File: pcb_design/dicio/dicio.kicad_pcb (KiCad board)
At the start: 2 copper layers, 93 x 93 mm, 88 parts, among them J1 USB_OTG, J2 Conn_01x06_Female, J3 Screw_Terminal_01x06, J4 Screw_Terminal_01x11, J5 Conn_02x03_Odd_Even, J6 Screw_Terminal_01x05, J7 Screw_Terminal_01x09, P1 USB_C_Plug_USB2.0, SW1 SW_SPST, SW2 SW_SPST, SW3 SW_DIP_x08, U1 FT232RL, U2 MCP2542FD, U3 dsPIC33EP512MC806, U4 TPS737, U5 PCA9670, U6 TPS61040, U7 RP604x, U8 gloxinia_connector_small, Y1 Crystal_GND24

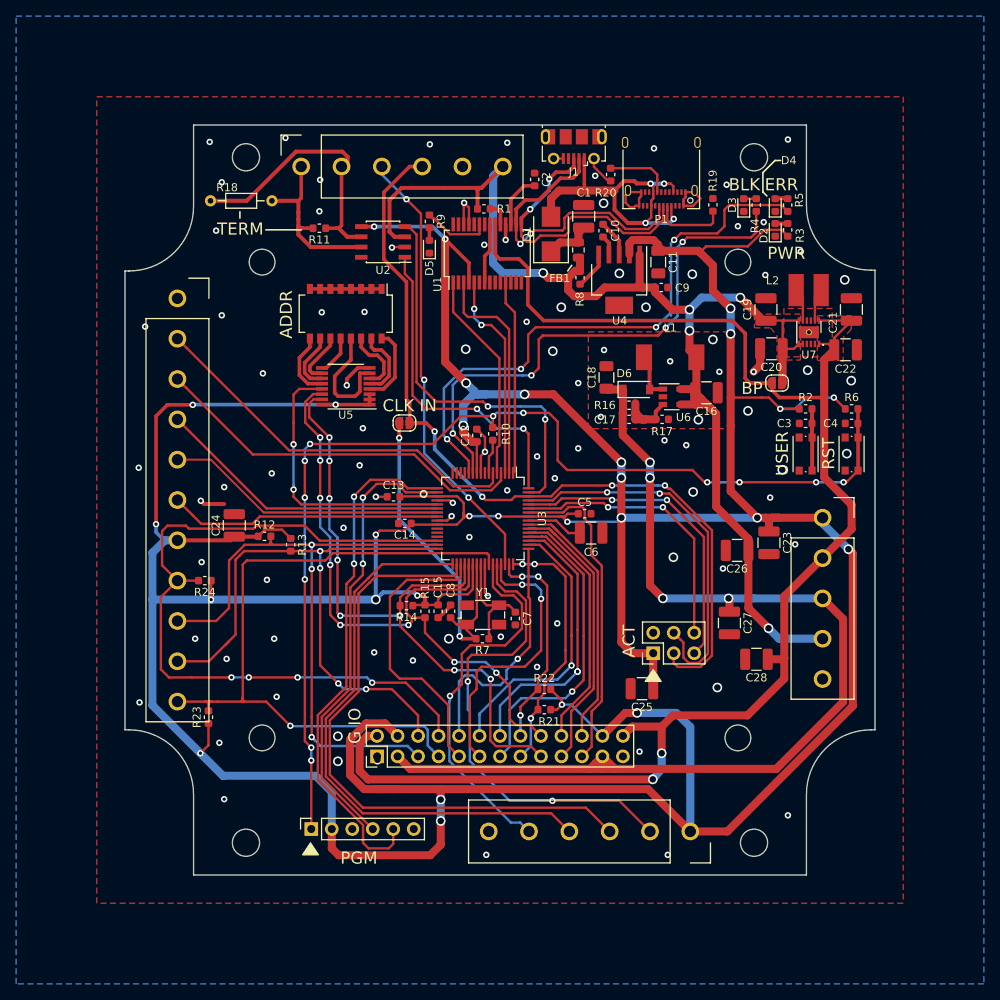
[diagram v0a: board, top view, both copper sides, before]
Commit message: New dicio design.
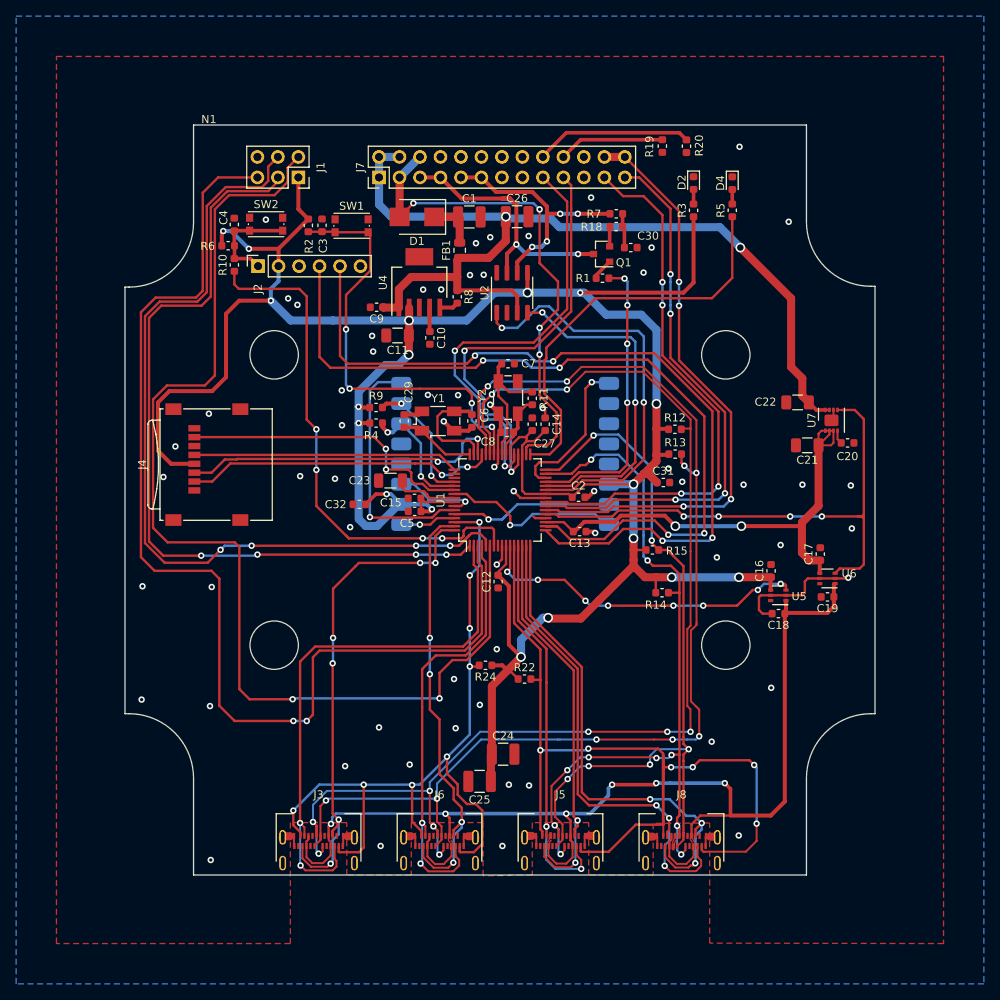
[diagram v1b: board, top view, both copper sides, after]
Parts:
- removed C28: 10uF, Capacitor_SMD:C_1210_3225Metric
- removed D3, D5: LED, LED_SMD:LED_0603_1608Metric
- removed D6: MBR0530, Diode_SMD:D_SOD-123
- removed H1, H2, H3, H4: MountingHole, MountingHole:MountingHole_3.2mm_M3
- removed JP1: Jumper_NC_Small, Jumper:SolderJumper-2_P1.3mm_Open_RoundedPad1.0x1.5mm
- removed JP2: Jumper, Jumper:SolderJumper-2_P1.3mm_Open_RoundedPad1.0x1.5mm
- removed L1: 10uH, custom_footprints:L_6.5mmx4.5mm_Bourns
- removed L2: 2.2uH, custom_footprints:L_L4mm_D4mm_H1.8mm
- removed P1: USB_C_Plug_USB2.0, custom_footprints:USB_C_Receptacle_Amphenol_12401832E402A
- removed R16: 1.8M, Capacitor_SMD:C_0603_1608Metric
- removed R17: 205k, Capacitor_SMD:C_0603_1608Metric
- removed R21, R23: 4.9k, Resistor_SMD:R_0603_1608Metric
- removed SW3: SW_DIP_x08, Button_Switch_SMD:SW_DIP_SPSTx08_Slide_Omron_A6H-8101_W6.15mm_P1.27mm
- removed U8: gloxinia_connector_small, Connector_PinHeader_2.54mm:PinHeader_2x13_P2.54mm_Vertical
- added C29: 20pF, Capacitor_SMD:C_0603_1608Metric, F.Cu at (73.1, 75.2)
- added C30: 4.7nF, Capacitor_SMD:C_0603_1608Metric, F.Cu at (101.2, 53.7)
- added C31: 0.1uF, Capacitor_SMD:C_0603_1608Metric, F.Cu at (105.2, 82.8)
- added C32: 0.1uF, Capacitor_SMD:C_0603_1608Metric, F.Cu at (67.6, 85.5)
- added J8: USB_C_Receptacle, custom_footprints:USB_C_Receptacle_Amphenol_12401861XX12A, F.Cu at (107.5, 127.9)
- added Q1: Q_NMOS_GSD, Package_TO_SOT_SMD:SOT-23, F.Cu at (97.6, 54.5)
- added Y2: Crystal_GND24, Crystal:Crystal_SMD_Abracon_ABM3B-4Pin_5.0x3.2mm, F.Cu at (86.0, 72.3)
- C16: value 10uF -> 1uF; footprint Capacitor_SMD:C_1210_3225Metric -> Capacitor_SMD:C_0603_1608Metric
- C17: value 4.7pF -> 1uF
- C18: value 1uF -> 0.1uF; footprint Capacitor_SMD:C_1206_3216Metric -> Capacitor_SMD:C_0603_1608Metric
- C19, C27: value 10uF -> 0.1uF; footprint Capacitor_SMD:C_1210_3225Metric -> Capacitor_SMD:C_0603_1608Metric
- C20: value 10uF -> 1nF; footprint Capacitor_SMD:C_1210_3225Metric -> Capacitor_SMD:C_0603_1608Metric
- C21, C22: value 22uF -> 4.7uF; footprint Capacitor_SMD:C_1210_3225Metric -> Capacitor_SMD:C_1206_3216Metric
- C23: footprint Capacitor_SMD:C_1210_3225Metric -> Capacitor_SMD:C_1206_3216Metric
- C6: value 10uF -> 20pF; footprint Capacitor_SMD:C_1210_3225Metric -> Capacitor_SMD:C_0603_1608Metric
- C7, C8: value 10pF -> 20pF
- J1: value USB_OTG -> Conn_02x03_Counter_Clockwise; footprint Connector_USB:USB_Micro-B_Molex-105017-0001 -> Connector_PinSocket_2.54mm:PinSocket_2x03_P2.54mm_Vertical
- J3: value Screw_Terminal_01x06 -> USB_C_Receptacle; footprint custom_footprints:TB003-500-06 -> custom_footprints:USB_C_Receptacle_Amphenol_12401861XX12A
- J4: value Screw_Terminal_01x11 -> Micro_SD_Card; footprint custom_footprints:TB003-500-11 -> Connector_Card:microSD_HC_Wuerth_693072010801
- J5: value Conn_02x03_Odd_Even -> USB_C_Receptacle; footprint Connector_PinHeader_2.54mm:PinHeader_2x03_P2.54mm_Vertical -> custom_footprints:USB_C_Receptacle_Amphenol_12401861XX12A
- J6: value Screw_Terminal_01x05 -> USB_C_Receptacle; footprint custom_footprints:TB003-500-05 -> custom_footprints:USB_C_Receptacle_Amphenol_12401861XX12A
- J7: value Screw_Terminal_01x09 -> Conn_02x13_Odd_Even; footprint custom_footprints:TB003-500-06 -> Connector_PinHeader_2.54mm:PinHeader_2x13_P2.54mm_Vertical
- N1: footprint custom_footprints:Enclosure-Hammond-1554LA -> custom_footprints:Enclosure-Gloxinia2
- R1: value 10k -> 1k
- R11: value 120 -> 1M
- R18: value 120R -> 60R; footprint Resistor_THT:R_Axial_DIN0204_L3.6mm_D1.6mm_P7.62mm_Horizontal -> Resistor_SMD:R_0603_1608Metric
- R4, R9: value 750 -> 100k
- R7: value 1M -> 60R
- SW1, SW2: footprint Button_Switch_SMD:SW_SPST_KMR2 -> Button_Switch_SMD:SW_Push_1P1T_NO_CK_KMR2
- U1: value FT232RL -> dsPIC33EP256MU806; footprint Package_SO:SSOP-28_5.3x10.2mm_P0.65mm -> Package_QFP:TQFP-64_10x10mm_P0.5mm
- U3: value dsPIC33EP512MC806 -> S70FL01GS; footprint Package_QFP:TQFP-64_10x10mm_P0.5mm -> custom_footprints:SOIC-16_25.75x18.75mm_P2.5mm; moved to B.Cu
- U5: value PCA9670 -> SiP32431; footprint Package_SO:TSSOP-16_4.4x5mm_P0.65mm -> Package_TO_SOT_SMD:SOT-363_SC-70-6
- U6: value TPS61040 -> SiP32431; footprint Package_TO_SOT_SMD:SOT-23-5 -> Package_TO_SOT_SMD:SOT-363_SC-70-6
- U7: value RP604x -> ADM7170; footprint custom_footprints:DFN_12_Pin_2.7x3mm_P0.5mm -> Package_CSP:LFCSP-8-1EP_3x3mm_P0.5mm_EP1.45x1.74mm
- moved J7 85.2 mm to (70.0, 45.0), turned to 90 degrees
- moved J3 84.9 mm to (62.5, 127.9)
- moved C4 80.4 mm to (52.0, 50.8), turned to 90 degrees
- moved R6 79.9 mm to (51.3, 53.5)
- moved SW2 78.0 mm to (56.0, 50.8), turned to 0 degrees
- moved J2 70.1 mm to (55.0, 56.0)
- moved R2 65.7 mm to (61.2, 51.0), turned to -90 degrees
- moved C3 64.8 mm to (62.9, 50.9), turned to 90 degrees
- moved SW1 63.0 mm to (66.6, 51.0), turned to 0 degrees
- moved U5 59.6 mm to (119.5, 96.8)
- moved J6 56.6 mm to (77.5, 127.9), turned to 0 degrees
- moved R7 55.2 mm to (99.4, 49.5), turned to 0 degrees
- moved R4 54.3 mm to (69.6, 75.5), turned to 0 degrees
- moved R12 52.6 mm to (106.7, 76.2)
- moved R18 50.4 mm to (99.4, 51.1), turned to 180 degrees
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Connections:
- net /~MCLR renamed /~{MCLR}
- C12 pad 1: +3V3 -> GND
- C12 pad 2: GND -> +3V3
- C13 pad 2: +3V3 -> VDDA
- C14 pad 1: +3V3 -> GND
- C14 pad 2: GND -> +3V3
- C16 pad 1: VBUS -> +3V3
- C17 pad 1: +12V -> VDDA
- C17 pad 2: Net-(C17-Pad2) -> GND
- C18 pad 1: +12V -> /S_PS
- C19 pad 1: VBUS -> /S_PS
- C2 pad 1: GND -> +3V3
- C2 pad 2: Net-(C2-Pad2) -> GND
- C20 pad 1: VBUS -> Net-(C20-Pad1)
- C21 pad 1: +5V -> VDDA
- C22 pad 1: +5V -> VBUS
- C23 pad 1: +3V3 -> /VCAP
- C27 pad 1: +12V -> +3V3
- C3 pad 1: Net-(C3-Pad1) -> /BTN
- C6 pad 1: Net-(C6-Pad1) -> GND
- C6 pad 2: GND -> /SOSC1
- C7 pad 2: Net-(C7-Pad2) -> /OSC2
- C8 pad 2: /CLK_IN -> /OSC1
- J1 pad 1: /V_USBC -> +3V3
- J1 pad 2: /D- -> /U1RX
- J1 pad 3: /D+ -> /~{U1RTS}
- J1 pad 4: Net-(J1-Pad4) -> /~{U1CTS}
- J1 pad 5: GND -> /U1TX
- J2 pad 6: /PGM -> unconnected-(J2-Pad6)
- J4 pad 1: GND -> unconnected-(J4-Pad1)
- J4 pad 2: /SCK2 -> /~{CS_SD}
- J4 pad 3: /SDO2 -> /MOSI1
- J4 pad 4: /SDI2 -> +3V3
- J4 pad 5: /~CS2_1 -> /SCK1
- J4 pad 6: /~CS2_2 -> GND
- J4 pad 7: +3V3 -> /MISO1
- J4 pad 8: /~INT2 -> unconnected-(J4-Pad8)
- J4 pad 9: /SDA2 -> GND
- J7 pad 1: +3V3 -> VBUS
- J7 pad 2: /U1RX -> VBUS
- J7 pad 3: /U1TX -> /V_USBC
- J7 pad 4: /~U1RTS -> VBUS
- J7 pad 5: /~U1CTS -> /CAN_H
- J7 pad 6: GND -> /V_USBC
- R1 pad 1: /~RST_FTDI -> Net-(Q1-Pad1)
- R1 pad 2: VBUS -> /TERM
- R10 pad 1: Net-(R10-Pad1) -> /~{MCLR_w}
- R11 pad 1: /CAN_L -> /OSC2
- R11 pad 2: /CAN_H -> /OSC1
- R18 pad 1: /CAN_L -> Net-(C30-Pad1)
- R18 pad 2: /CAN_H -> Net-(Q1-Pad2)
- R19 pad 1: Net-(P1-PadA5) -> /VCONN
- R2 pad 2: Net-(C3-Pad1) -> /BTN
- R20 pad 2: Net-(P1-PadB5) -> /CC1
- R22 pad 2: /~INT1 -> /~{INT1}
- R24 pad 2: /~INT2 -> /~{INT2}
- R4 pad 1: /BLINK -> +3V3
- R4 pad 2: Net-(D3-Pad2) -> /~{SQICS1}
- R7 pad 1: Net-(C7-Pad2) -> /CAN_L
- R7 pad 2: /CLK_IN -> Net-(C30-Pad1)
- R9 pad 1: Net-(R9-Pad1) -> +3V3
- R9 pad 2: Net-(D5-Pad2) -> /~{SQICS0}
- SW1 pad 2: Net-(C3-Pad1) -> /BTN
- U1 pad 1: /MCU_RXD -> /~{U1RTS}
- U1 pad 10: Net-(U1-Pad10) -> +3V3
- U1 pad 11: /MCU_~RTS -> /S_PS_SW
- U1 pad 12: Net-(U1-Pad12) -> /~{INT1}
- U1 pad 13: Net-(U1-Pad13) -> /OW2
- U1 pad 14: Net-(U1-Pad14) -> /AS2
- U1 pad 15: /D+ -> /OW4
- U1 pad 16: /D- -> /AS4
- U1 pad 17: Net-(C2-Pad2) -> /PGC
- U1 pad 18: GND -> /PGD
- U1 pad 19: /~RST_FTDI -> VDDA
- U1 pad 2: Net-(U1-Pad2) -> /OW1
- U1 pad 20: +5V -> GND
- U1 pad 21: GND -> /EN_VA
- U1 pad 22: Net-(U1-Pad22) -> /SYNC
- U1 pad 23: Net-(R9-Pad1) -> /CAN_C2
- U1 pad 24: (no net) -> /CAN_C1
- U1 pad 26: GND -> +3V3
- U1 pad 27: Net-(U1-Pad27) -> /C1TX
- U1 pad 28: Net-(U1-Pad28) -> /C1RX
- U1 pad 3: /MCU_~CTS -> /U1TX
- U1 pad 4: +3V3 -> /OW3
- U1 pad 5: /MCU_TXD -> /~{U1CTS}
- U1 pad 6: Net-(U1-Pad6) -> /U1RX
- U1 pad 7: GND -> /~{MCLR_w}
- U1 pad 8: (no net) -> unconnected-(U1-Pad8)
- U1 pad 9: Net-(U1-Pad9) -> GND
- U3 pad 1: /MCU_~RTS -> /~{HOLD}
- U3 pad 10: +3V3 -> GND
- U3 pad 11: /BLINK -> unconnected-(U3-Pad11)
- U3 pad 12: /ERR -> unconnected-(U3-Pad12)
- U3 pad 13: Net-(U3-Pad13) -> unconnected-(U3-Pad13)
- U3 pad 14: Net-(U3-Pad14) -> +3V3
- U3 pad 15: Net-(U3-Pad15) -> /SI
- U3 pad 16: Net-(U3-Pad16) -> /SQICLK
- U3 pad 2: /MCU_~CTS -> +3V3
- U3 pad 3: /MCU_TXD -> /~{RESET_M}
- U3 pad 4: /SDO2 -> unconnected-(U3-Pad4)
- U3 pad 5: /MCU_RXD -> unconnected-(U3-Pad5)
- U3 pad 6: /SCK2 -> /~{SQICS1}
- U3 pad 7: Net-(R10-Pad1) -> /~{SQICS0}
- U3 pad 8: Net-(U3-Pad8) -> /SO
- U3 pad 9: GND -> /~{WP}
- U5 pad 1: +3V3 -> /S_PS
- U5 pad 2: +3V3 -> GND
- U5 pad 3: +3V3 -> /S_PS_SW
- U5 pad 4: Net-(SW3-Pad16) -> +3V3
- U5 pad 5: Net-(SW3-Pad15) -> GND
- U5 pad 6: Net-(SW3-Pad14) -> unconnected-(U5-Pad6)
- U6 pad 1: Net-(D6-Pad2) -> /S_PS
- U6 pad 3: Net-(C17-Pad2) -> /EN_VA
- U6 pad 4: VBUS -> VDDA
- U6 pad 5: VBUS -> GND
- U7 pad 1: VBUS -> VDDA
- U7 pad 2: VBUS -> VDDA
- U7 pad 3: GND -> VDDA
- U7 pad 4: GND -> Net-(C20-Pad1)
- U7 pad 5: GND -> /EN_VA
- U7 pad 6: +5V -> GND
- U7 pad 7: +5V -> VBUS
- U7 pad 8: Net-(L2-Pad2) -> VBUS
- Y1 pad 1: /CLK_IN -> /SOSC2
- Y1 pad 3: Net-(C7-Pad2) -> /SOSC1
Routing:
- net +3V3: track 606.6 -> 342.9 mm, vias 29 -> 18
- net +5V: track 190.2 -> 0.00 mm, vias 2 -> 0
- net /S_PS: track 0.00 -> 144.3 mm, vias 0 -> 6
- net +12V: track 130.5 -> 0.00 mm, vias 4 -> 0
- net /~{INT1}: track 0.00 -> 121.3 mm, vias 0 -> 6
- net /~{MCLR}: track 134.0 -> 12.8 mm, vias 12 -> 0
- net /~{U1CTS}: track 0.00 -> 107.3 mm, vias 0 -> 4
- net /CLK: track 104.0 -> 0.00 mm, vias 4 -> 0
- net /~{U1RTS}: track 0.00 -> 98.7 mm, vias 0 -> 4
- net /~{INT2}: track 0.00 -> 96.3 mm, vias 0 -> 8
- net /~INT2: track 96.2 -> 0.00 mm, vias 4 -> 0
- net /~RST2: track 88.7 -> 0.00 mm, vias 1 -> 0
- net /U1RX: track 58.7 -> 136.8 mm
- net /~U1RTS: track 71.0 -> 0.00 mm
- net /SDA2: track 79.4 -> 150.2 mm, vias 3 -> 10
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- added copper zone on F.Cu, net /S_PS
- removed copper zone on F.Cu, net +5V
- removed copper zone on F.Cu, net VBUS
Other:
- outline, holes or cut-outs redrawn
- net class Default removed
- board text removed: "12V"
- board text removed: "3.3V"
- board text removed: "5V"
- board text removed: "ACT"
- board text removed: "ADDR"
- board text removed: "BLK"
- board text removed: "BP"
- board text removed: "CH"
- board text removed: "CL"
- board text removed: "CLK"
- board text removed: "CLK IN"
- board text removed: "ERR"
- board text removed: "G IO"
- board text removed: "GND"
- board text removed: "IO"
- board text removed: "PGM"
- board text removed: "PWR"
- board text removed: "RST"
- board text removed: "RX"
- board text removed: "Rev. 4"
- board text removed: "SCK"
- board text removed: "SCL"
- board text removed: "SDA"
- board text removed: "SDI"
- board text removed: "SDO"
- board text removed: "TERM"
- board text removed: "TX"
- board text removed: "USER"
- board text removed: "VB"
- board text removed: "dicio"
- board text removed: "gloxinia system"
- board text removed: "~CS1"
- board text removed: "~CS2"
- board text removed: "~CTS"
- board text removed: "~INT"
- board text removed: "~RST"
- board text removed: "~RTS"
